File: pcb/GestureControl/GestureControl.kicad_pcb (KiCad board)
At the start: 4 copper layers, 214.8 x 54.6 mm, 157 parts, among them J1 Conn_01x04_I2I-LCD, J10 EXTERN I2C, J11 Conn_01x02, J12 Conn_01x02, J13 690367291076, J14 690367291076, J15 690367291076, J16 690367291076, J17 Conn_01x01, J18 Conn_01x01, J19 Conn_01x01, J2 BATT, J20 690367291076, J21 690367291076, J3 Conn_01x08, J4 Conn_01x06, J5 Conn_01x10, J6 Conn_01x08, J7 FTDI, J8 Conn_01x06, J9 UART, SW1 SW1, SW2 SW2, U1 AP5100_3.3, U2 AP5100_3.3, U3 VL53L3CXV0DH_1, U4 VL53L3CXV0DH_1, U5 VL53L3CXV0DH_1, U6 STM32L151RETx, U7 STM32F401RETx, U8 VL53L3CXV0DH_1, Y1 8MHz, Y2 32kHz

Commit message: cleanup
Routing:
- net GND: track 409.6 -> 408.3 mm
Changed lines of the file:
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@@
     (thickness 1.6)
     (drawings 259)
-    (tracks 1824)
+    (tracks 1822)
     (zones 0)
     (modules 157)
@@
   (segment (start 140.716 124.333) (end 145.796 124.333) (width 1) (layer GND) (net 1))
   (segment (start 145.796 124.333) (end 145.796 135.128) (width 1) (layer GND) (net 1))
-  (segment (start 140.857002 135.128) (end 140.716 135.269002) (width 1) (layer GND) (net 1))
   (segment (start 145.796 135.128) (end 140.857002 135.128) (width 1) (layer GND) (net 1))
-  (segment (start 140.716 135.269002) (end 140.716 136.398) (width 1) (layer GND) (net 1))
   (segment (start 183.896 124.333) (end 183.896 133.613318) (width 1) (layer GND) (net 1))
   (segment (start 183.896 133.613318) (end 183.896 135.763) (width 1) (layer GND) (net 1))

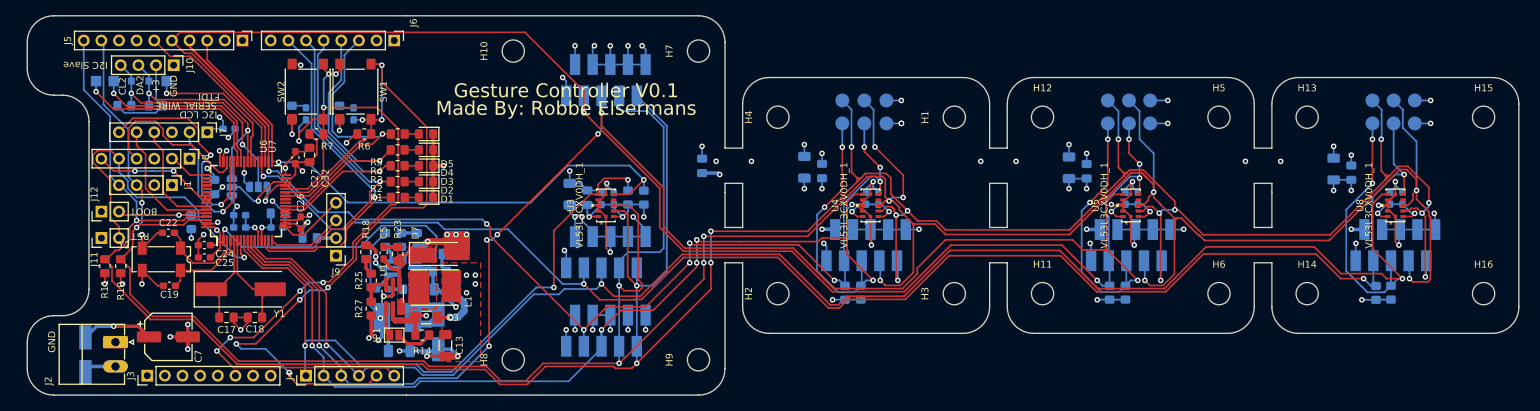
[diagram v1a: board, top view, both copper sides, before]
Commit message: add feedback PCB
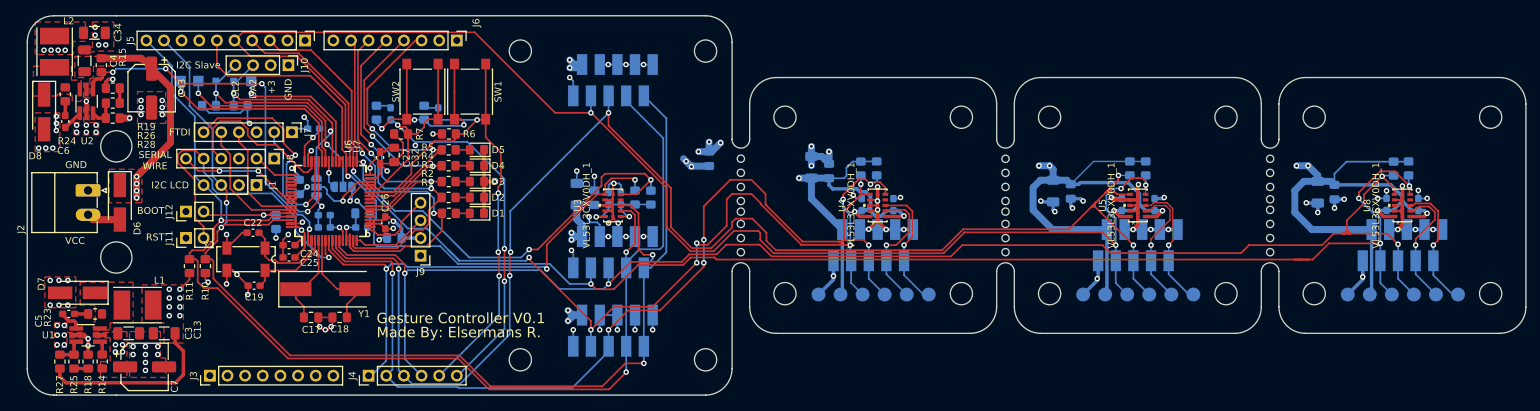
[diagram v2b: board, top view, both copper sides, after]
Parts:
- removed JP1, JP4: SolderJumper_2_Open, Jumper:SolderJumper-2_P1.3mm_Open_Pad1.0x1.5mm
- added C43: 10µ, Capacitor_SMD:CP_Elec_6.3x5.4, F.Cu at (59.4, 113.8)
- added REF**: MountingHole_4.5mm, MountingHole:MountingHole_4.5mm, F.Cu at (54.4, 138.2)
- added REF**: MountingHole_4.5mm, MountingHole:MountingHole_4.5mm, F.Cu at (54.4, 122.2)
- C34, C4, C6, D6, D8, L2, R15, R19, R24, R26, R28, U2: moved to F.Cu
- J13, J14, J15, J16, J20, J21: value 690367291076 -> WR-MM Female SMT Connector
- moved D8 65.0 mm to (44.0, 117.2)
- moved C34 63.4 mm to (51.2, 105.8)
- moved L2 62.5 mm to (45.5, 108.5), turned to 90 degrees
- moved C4 61.4 mm to (49.8, 109.9), turned to 90 degrees
- moved R15 57.1 mm to (52.2, 110.5), turned to -90 degrees
- moved R24 57.0 mm to (47.0, 114.7), turned to -90 degrees
- moved D7 52.5 mm to (48.8, 143.3), turned to 180 degrees
- moved C6 51.7 mm to (47.0, 118.6), turned to -90 degrees
- moved U2 51.5 mm to (50.1, 115.7), turned to 90 degrees
- moved R19 49.0 mm to (53.8, 113.8), turned to 180 degrees
- moved R14 46.2 mm to (52.3, 153.1), turned to 90 degrees
- moved C5 46.2 mm to (47.5, 146.3), turned to 180 degrees
- moved R26 46.0 mm to (53.8, 116.0), turned to 0 degrees
- moved R27 45.5 mm to (46.2, 153.2)
- moved R23 44.4 mm to (51.3, 146.3), turned to 180 degrees
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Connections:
- J13 pad 2: SCL1 -> SDA1
- J13 pad 4: SDA1 -> SCL1
- J14 pad 2: SCL1 -> SDA1
- J14 pad 4: SDA1 -> SCL1
- J15 pad 2: SCL1 -> SDA1
- J15 pad 4: SDA1 -> SCL1
- J16 pad 2: SCL1 -> SDA1
- J16 pad 4: SDA1 -> SCL1
- J20 pad 2: SCL1 -> SDA1
- J20 pad 4: SDA1 -> SCL1
- J21 pad 2: SCL1 -> SDA1
- J21 pad 4: SDA1 -> SCL1
- J3 pad 1: (no net) -> unconnected-(J3-Pad1)
- J3 pad 2: (no net) -> unconnected-(J3-Pad2)
- J3 pad 3: (no net) -> unconnected-(J3-Pad3)
- J3 pad 8: (no net) -> unconnected-(J3-Pad8)
- J5 pad 1: (no net) -> unconnected-(J5-Pad1)
- J5 pad 2: (no net) -> unconnected-(J5-Pad2)
- J6 pad 1: (no net) -> unconnected-(J6-Pad1)
- J6 pad 2: (no net) -> unconnected-(J6-Pad2)
- J6 pad 8: (no net) -> unconnected-(J6-Pad8)
- R14 pad 2: Net-(JP1-Pad1) -> BUCK_33_EN
- R15 pad 2: Net-(JP4-Pad1) -> BUCK_5_EN
- U3 pad 8: (no net) -> unconnected-(U3-Pad8)
- U4 pad 8: (no net) -> unconnected-(U4-Pad8)
- U5 pad 8: (no net) -> unconnected-(U5-Pad8)
- U6 pad 20: (no net) -> unconnected-(U6-Pad20)
- U6 pad 21: (no net) -> unconnected-(U6-Pad21)
- U6 pad 24: (no net) -> unconnected-(U6-Pad24)
- U6 pad 25: (no net) -> unconnected-(U6-Pad25)
- U6 pad 37: (no net) -> unconnected-(U6-Pad37)
- U6 pad 38: (no net) -> unconnected-(U6-Pad38)
- U6 pad 50: (no net) -> unconnected-(U6-Pad50)
- U6 pad 51: (no net) -> unconnected-(U6-Pad51)
- U6 pad 52: (no net) -> unconnected-(U6-Pad52)
- U6 pad 53: (no net) -> unconnected-(U6-Pad53)
- U6 pad 54: (no net) -> unconnected-(U6-Pad54)
- U6 pad 56: (no net) -> unconnected-(U6-Pad56)
- U6 pad 57: (no net) -> unconnected-(U6-Pad57)
- U7 pad 20: (no net) -> unconnected-(U7-Pad20)
- U7 pad 21: (no net) -> unconnected-(U7-Pad21)
- U7 pad 24: (no net) -> unconnected-(U7-Pad24)
- U7 pad 25: (no net) -> unconnected-(U7-Pad25)
- U7 pad 37: (no net) -> unconnected-(U7-Pad37)
- U7 pad 38: (no net) -> unconnected-(U7-Pad38)
- U7 pad 50: (no net) -> unconnected-(U7-Pad50)
- U7 pad 51: (no net) -> unconnected-(U7-Pad51)
- U7 pad 52: (no net) -> unconnected-(U7-Pad52)
- U7 pad 53: (no net) -> unconnected-(U7-Pad53)
- U7 pad 54: (no net) -> unconnected-(U7-Pad54)
- U7 pad 56: (no net) -> unconnected-(U7-Pad56)
- U7 pad 57: (no net) -> unconnected-(U7-Pad57)
- U8 pad 8: (no net) -> unconnected-(U8-Pad8)
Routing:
- net SDA1: track 454.5 -> 357.9 mm, vias 14 -> 7
- net SCL1: track 437.5 -> 362.7 mm, vias 17 -> 6
- net GND: track 408.3 -> 356.7 mm, vias 76 -> 125
- net XSHUT_3: track 255.0 -> 207.3 mm, vias 5 -> 4
- net +3V3: track 700.3 -> 744.9 mm, vias 48 -> 41
- net SW_2: track 117.5 -> 77.9 mm, vias 7 -> 4
- net VCC: track 99.5 -> 60.6 mm, vias 3 -> 8
- net SW_1: track 115.0 -> 77.4 mm, vias 7 -> 4
- net /OUT3.3: track 34.6 -> 0.00 mm
- net XSHUT_2: track 239.2 -> 207.0 mm, vias 9 -> 6
- net XSHUT_1: track 170.5 -> 142.5 mm, vias 7 -> 6
- net XSHUT_0: track 93.0 -> 74.0 mm
- net GPIOI_1: track 174.9 -> 156.3 mm, vias 9 -> 8
- net +5V: track 108.2 -> 122.4 mm, vias 2 -> 5
- net /OUT5.0: track 13.8 -> 0.00 mm
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- added copper zone on In2.Cu, net +3V3
- added copper zone on F.Cu, net +5V
- added copper zone on In2.Cu, net +5V
- added copper zone on F.Cu, net /OUT5.0
- added copper zone on F.Cu, net GND
- added copper zone on In1.Cu, net GND
- added copper zone on F.Cu, net VCC
- removed copper zone on PWR, net +3V3
- removed copper zone on GND, net GND
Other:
- board size 214.8 x 54.6 mm -> 215.8 x 54.6 mm
- net class Default removed
- net class PWR removed
- board text added: "3V3"
- board text added: "G0"
- board text added: "G1"
- board text added: "G2"
- board text added: "G3"
- board text added: "LED1"
- board text added: "LED2"
- board text added: "LED3"
- board text added: "LED4"
- board text added: "LED5"
- board text added: "Made By: Elsermans R."
- board text added: "SW1"
- board text added: "SW2"
- board text added: "VCC"
- board text added: "XS3"
- board text removed: "D1"
- board text removed: "D2"
- board text removed: "D3"
- board text removed: "D4"
- board text removed: "D5"
- board text removed: "GND 3V3"
- board text removed: "GP0"
- board text removed: "GP1"
- board text removed: "GP2"
- board text removed: "Made By: Robbe Elsermans"
- board text removed: "SCL XSHUT"
- board text removed: "SDA GPIOI"
